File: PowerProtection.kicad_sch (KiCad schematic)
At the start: 17 parts, among them U1 LM76202QPWPRQ1

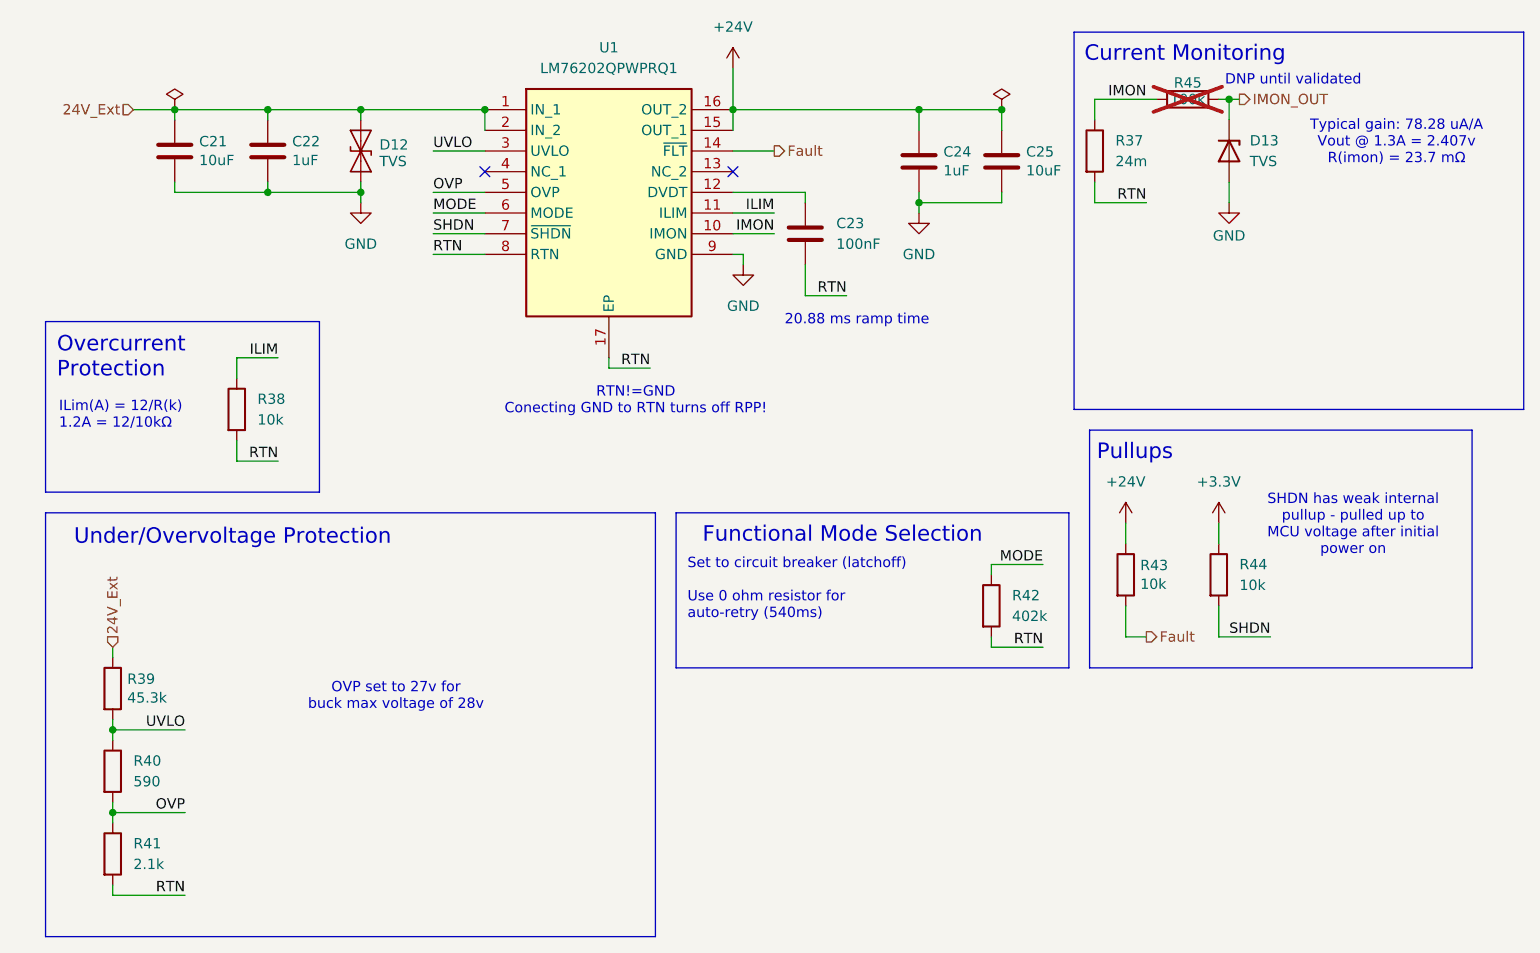
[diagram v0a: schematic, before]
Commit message: changed rpp circuit to match vcu
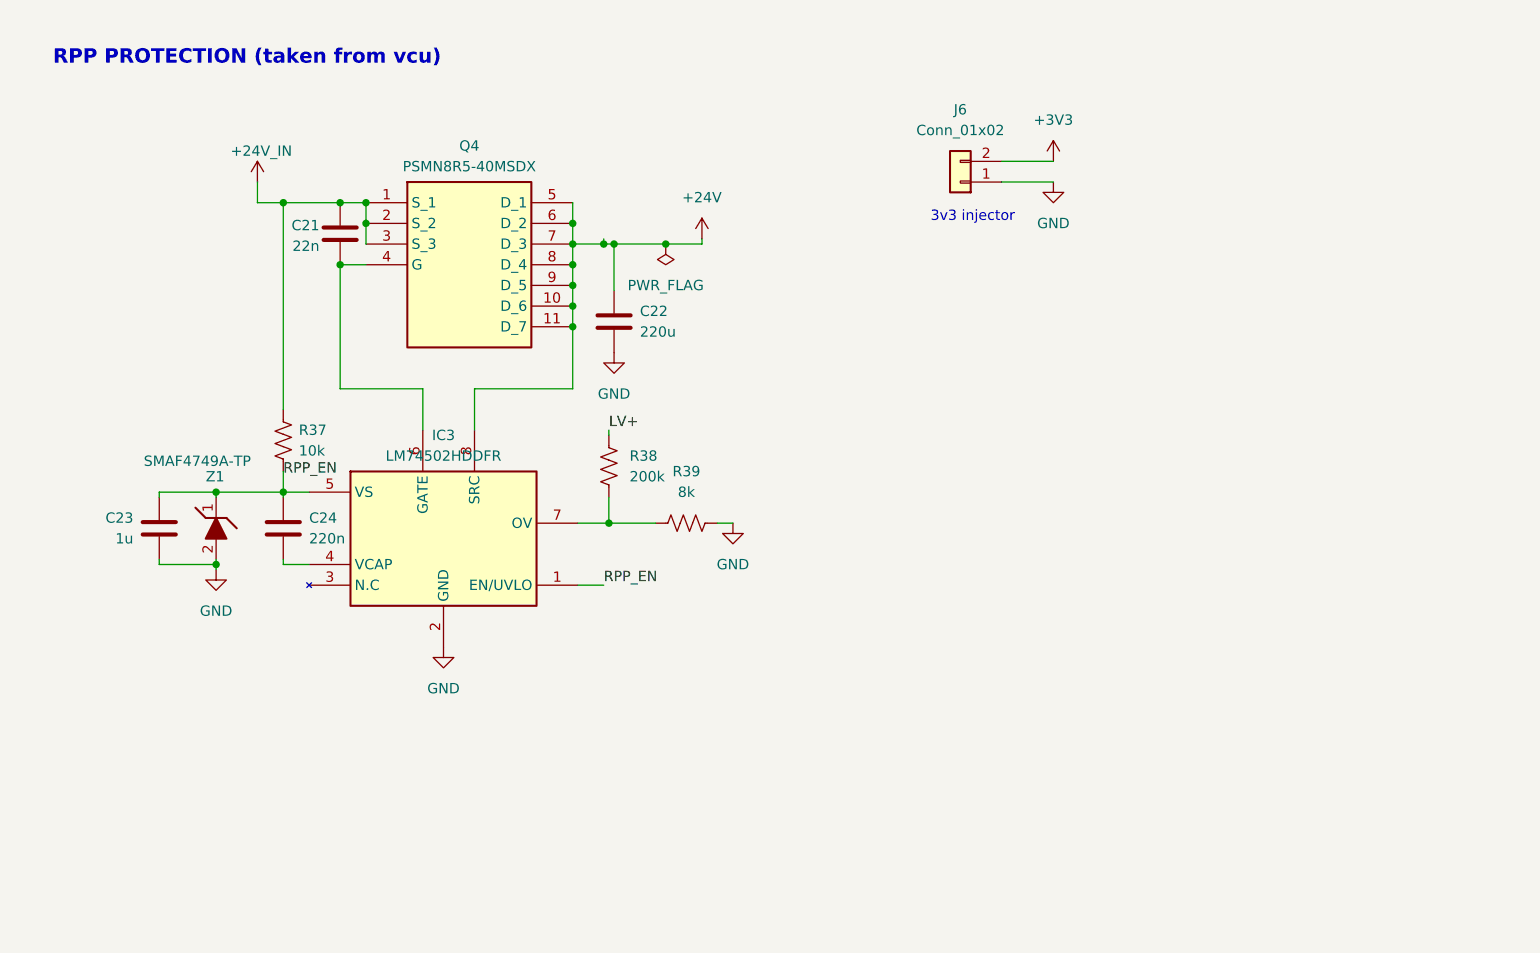
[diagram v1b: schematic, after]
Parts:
- removed C25: 10uF, Capacitor_SMD:C_0805_2012Metric_Pad1.18x1.45mm_HandSolder, symbol Device:C
- removed D12: TVS, Diode_SMD:D_SOD-323_HandSoldering, symbol Diode:SD12_SOD323
- removed D13: TVS, Diode_SMD:D_SOD-123F, symbol Device:D_Zener
- removed R37: 24m, Resistor_SMD:R_0603_1608Metric_Pad0.98x0.95mm_HandSolder, symbol Device:R
- removed R38, R43, R44: 10k, Resistor_SMD:R_0603_1608Metric_Pad0.98x0.95mm_HandSolder, symbol Device:R
- removed R39: 45.3k, Resistor_SMD:R_0603_1608Metric_Pad0.98x0.95mm_HandSolder, symbol Device:R
- removed R40: 590, Resistor_SMD:R_0603_1608Metric_Pad0.98x0.95mm_HandSolder, symbol Device:R
- removed R41: 2.1k, Resistor_SMD:R_0603_1608Metric_Pad0.98x0.95mm_HandSolder, symbol Device:R
- removed R42: 402k, Resistor_SMD:R_0603_1608Metric_Pad0.98x0.95mm_HandSolder, symbol Device:R
- removed R45: 100k, Resistor_SMD:R_0603_1608Metric_Pad0.98x0.95mm_HandSolder, symbol Device:R
- removed U1: LM76202QPWPRQ1, UTSVT_Power:LM76202QPWPRQ1, symbol utsvt_power:LM76202QPWPRQ1
- added IC3: LM74502HDDFR, LM74502HDDFR:SOT65P280X110-8N, symbol UTSVT_ICs:LM74502HDDFR
- added J6: Conn_01x02, UTSVT_Connectors:Molex_Nano-Fit_105309-xx02_1x02_P2.50mm_Vertical, symbol Connector_Generic:Conn_01x02
- added Q4: PSMN8R5-40MSDX, PSMN8R5-40MSDX:BUK7M1780EX, symbol UTSVT_Power:PSMN8R5-40MSDX
- added R37: 10k, Resistor_SMD:R_0603_1608Metric, symbol Device:R_US
- added R38: 200k, Resistor_SMD:R_0603_1608Metric, symbol Device:R_US
- added R39: 8k, Resistor_SMD:R_0603_1608Metric, symbol Device:R_US
- added Z1: SMAF4749A-TP, DO-221AC-2:SODFL5026X125N, symbol UTSVT_Power:SMAF4749A-TP
- C21: value 10uF -> 22n; footprint Capacitor_SMD:C_0805_2012Metric_Pad1.18x1.45mm_HandSolder -> Capacitor_SMD:C_0603_1608Metric; P/N GRM21BR61H106KE43K -> (none)
- C22: value 1uF -> 220u; footprint Capacitor_SMD:C_0603_1608Metric_Pad1.08x0.95mm_HandSolder -> Capacitor_SMD:C_0603_1608Metric; P/N MLASU168SB5105KTNA01 -> (none)
- C23: value 100nF -> 1u; footprint Capacitor_SMD:C_0603_1608Metric_Pad1.08x0.95mm_HandSolder -> Capacitor_SMD:C_0603_1608Metric; P/N MLASH168SB7104KTNA01 -> (none)
- C24: value 1uF -> 220n; footprint Capacitor_SMD:C_0603_1608Metric_Pad1.08x0.95mm_HandSolder -> Capacitor_SMD:C_0603_1608Metric; P/N MLASU168SB5105KTNA01 -> (none)
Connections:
- net +24V: now also C22.1, IC3.8 (SRC), Q4.10 (D_6), Q4.11 (D_7), Q4.5 (D_1), Q4.6 (D_2), Q4.7 (D_3), Q4.8 (D_4), Q4.9 (D_5); no longer C24.1
- net GND: now also C23.1, IC3.2 (GND), J6.1 (Pin_1), R39.2, Z1.2 (A); no longer C21.2, C24.2
- net 24V_Ext: no longer names the net of C21.1
- net 24V_Ext: now also IC3.6 (GATE), Q4.4 (G); no longer C22.1
- net RTN renamed RPP_EN
- net RPP_EN: now also C24.1, IC3.1 (EN/UVLO), IC3.5 (VS), R37.2, Z1.1 (K)
- new net: C24.2, IC3.4 (VCAP)
- new net: IC3.7 (OV), R38.2, R39.1
- new net +24V_IN: C21.2, Q4.1 (S_1), Q4.2 (S_2), Q4.3 (S_3), R37.1
- new net +3V3: J6.2 (Pin_2)
- new net LV+: R38.1
- no-connect marks 2 -> 0
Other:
- note added: "3v3 injector"
- note added: "RPP PROTECTION (taken from vcu)"
- note removed: "20.88 ms ramp time"
- note removed: "Current Monitoring"
- note removed: "DNP until validated"
- note removed: "Functional Mode Selection"
- note removed: "ILim(A) = 12/R(k) 1.2A = 12/10kΩ"
- note removed: "OVP set to 27v for buck max voltage of 28v"
- note removed: "Overcurrent Protection"
- note removed: "Pullups"
- note removed: "RTN!=GND Conecting GND to RTN turns off RPP!"
- note removed: "SHDN has weak internal pullup - pulled up to MCU voltage after initial power on"
- note removed: "Set to circuit breaker (latchoff) Use 0 ohm resistor for auto-retry (540ms)"
- note removed: "Typical gain: 78.28 uA/A Vout @ 1.3A = 2.407v R(imon) = 23.7 mΩ"
- note removed: "Under/Overvoltage Protection"
